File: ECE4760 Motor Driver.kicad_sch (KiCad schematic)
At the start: 48 parts, among them J1 IO, J100 Alternative Motor, J2 Motor / Power, J4 UART, U1 STM32G473V_B-C-E_Hx, U5 AP7361C-33FGE, U7 TPSM365R6, X1 48MHz

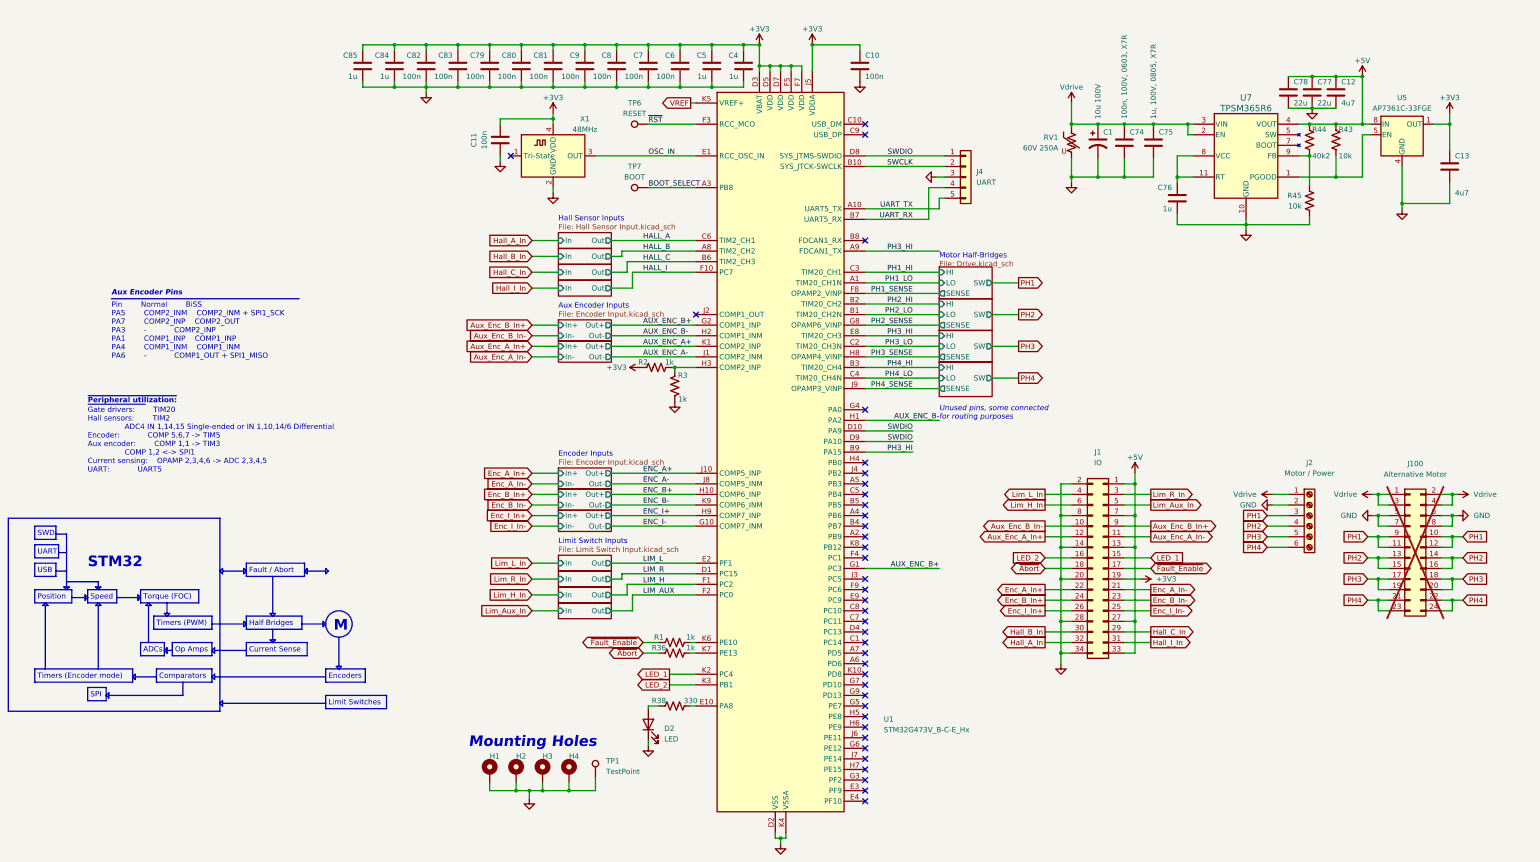
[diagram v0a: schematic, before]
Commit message: Ready for design review
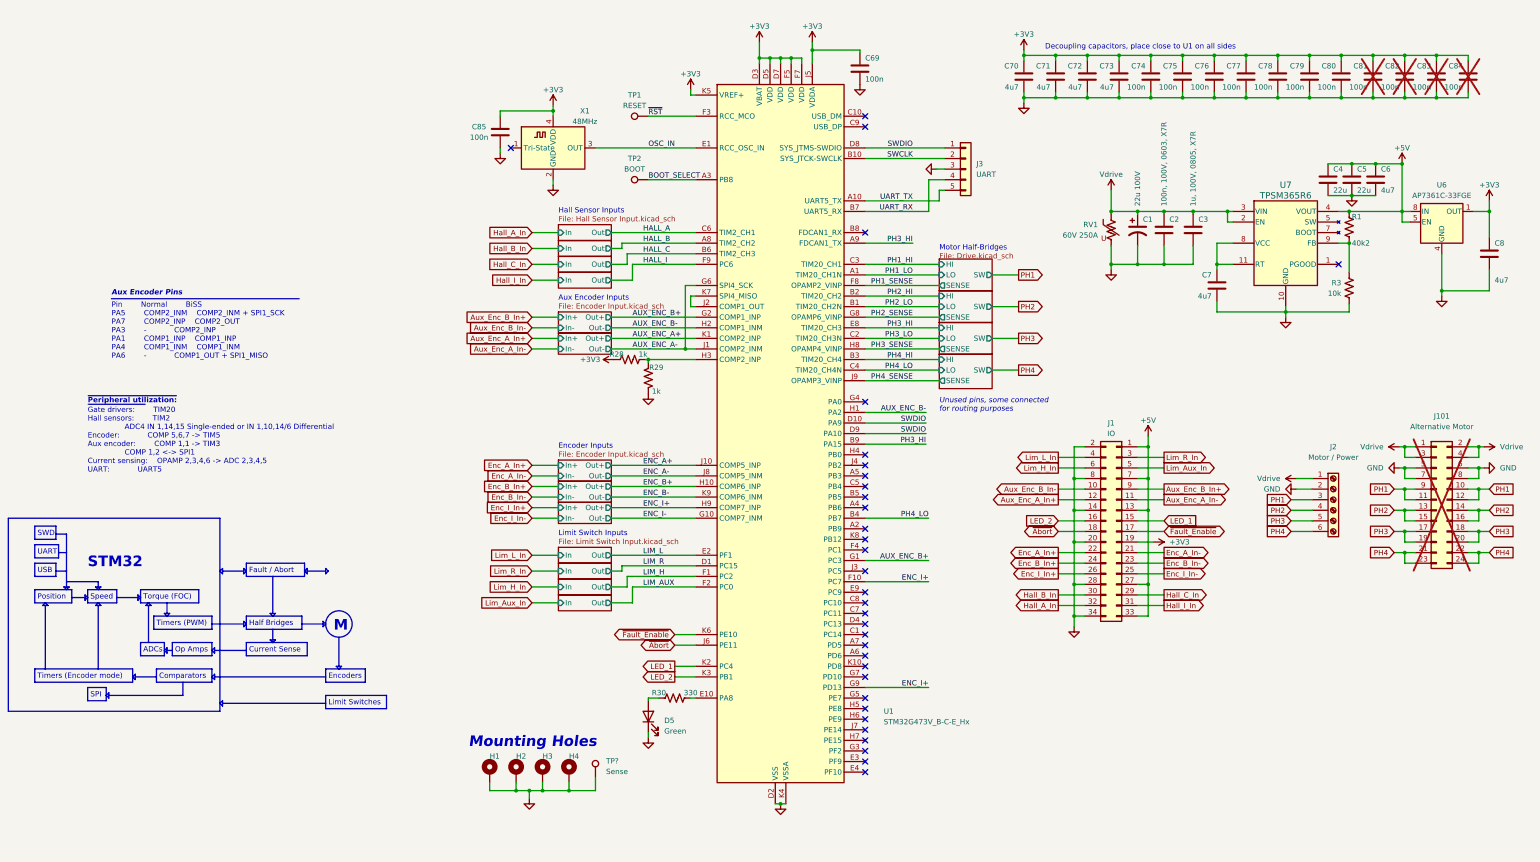
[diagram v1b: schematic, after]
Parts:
- removed R1, R36: 1k, Resistor_SMD:R_0402_1005Metric, symbol Device:R_US
- removed R43: 10k, Resistor_SMD:R_0402_1005Metric, symbol Device:R_US
- added C81, C82: 100n, Capacitor_SMD:C_0402_1005Metric, symbol Device:C
- C1: value 10u 100V -> 22u 100V
- C2: renamed from C74; DigiKey 490-3285-1-ND -> 490-13420-1-ND; LCSC (none) -> C161117
- C3: renamed from C75; LCSC (none) -> C5370002
- C4: renamed from C78; DigiKey (none) -> 490-GRM21BZ71A226ME15LCT-ND; LCSC (none) -> C907991
- C5: renamed from C77; DigiKey (none) -> 490-GRM21BZ71A226ME15LCT-ND; LCSC (none) -> C907991
- C6: renamed from C12; DigiKey (none) -> 490-GRM188Z71C475KE21DCT-ND; LCSC (none) -> C389010
- C69: renamed from C10; DigiKey 490-10700-1-ND -> 490-3261-1-ND; LCSC (none) -> C71629
- C7: renamed from C76; value 1u -> 4u7; DigiKey (none) -> 490-GRM188Z71C475KE21DCT-ND; LCSC (none) -> C389010
- C70: renamed from C5; value 1u -> 4u7; DigiKey (none) -> 490-GRM188Z71C475KE21DCT-ND; LCSC (none) -> C389010
- C71: renamed from C4; value 1u -> 4u7; DigiKey (none) -> 490-GRM188Z71C475KE21DCT-ND; LCSC (none) -> C389010
- C72: renamed from C85; value 1u -> 4u7; DigiKey (none) -> 490-GRM188Z71C475KE21DCT-ND; LCSC (none) -> C389010
- C73: renamed from C84; value 1u -> 4u7; DigiKey (none) -> 490-GRM188Z71C475KE21DCT-ND; LCSC (none) -> C389010
- C74: renamed from C79; DigiKey 490-10700-1-ND -> 490-3261-1-ND; LCSC (none) -> C71629
- C75: renamed from C80; DigiKey 490-10700-1-ND -> 490-3261-1-ND; LCSC (none) -> C71629
- C76: renamed from C81; DigiKey 490-10700-1-ND -> 490-3261-1-ND; LCSC (none) -> C71629
- C77: renamed from C9; DigiKey 490-10700-1-ND -> 490-3261-1-ND; LCSC (none) -> C71629
- C78: renamed from C8; DigiKey 490-10700-1-ND -> 490-3261-1-ND; LCSC (none) -> C71629
- C79: renamed from C7; DigiKey 490-10700-1-ND -> 490-3261-1-ND; LCSC (none) -> C71629
- C8: renamed from C13; DigiKey (none) -> 490-GRM188Z71C475KE21DCT-ND; LCSC (none) -> C389010
- C80: renamed from C6; DigiKey 490-10700-1-ND -> 490-3261-1-ND; LCSC (none) -> C71629
- C83: renamed from C82; DigiKey 490-10700-1-ND -> 490-3261-1-ND; LCSC (none) -> C71629; now not fitted; now left out of the parts list
- C84: renamed from C83; DigiKey 490-10700-1-ND -> 490-3261-1-ND; LCSC (none) -> C71629; now not fitted; now left out of the parts list
- C85: renamed from C11; DigiKey 490-10700-1-ND -> 490-3261-1-ND; LCSC (none) -> C71629
- D5: renamed from D2; value LED -> Green; DigiKey (none) -> 160-2018-1-ND; LCSC (none) -> C364563
- R1: renamed from R44; DigiKey 311-1.00KLRCT-ND -> 311-40.2KLRCT-ND; LCSC (none) -> C137983
- R28: renamed from R2; LCSC (none) -> C2935237
- R29: renamed from R3; LCSC (none) -> C2935237
- R3: renamed from R45; DigiKey 311-1.00KLRCT-ND -> 311-10.0KLRCT-ND; LCSC (none) -> C60490
- R30: renamed from R38; DigiKey (none) -> 311-330KLRCT-ND; LCSC (none) -> C138006
- TP1: renamed from TP6; now left out of the parts list
- TP2: renamed from TP7; now left out of the parts list
- TP?: renamed from TP1; value TestPoint -> Sense
- renumbered J100 to J101, J4 to J3, U5 to U6
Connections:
- net VREF is gone; now on net +3V3: U1.K5 (VREF+)
- net +3V3: now also C81.1, C82.1
- net +5V: now also U6.5 (EN)
- net AUX_ENC_A-: now also U1.G6 (PE12)
- net ENC_I+: now also U1.F10 (PC7), U1.G9 (PD13)
- net GND: now also C81.2, C82.2
- net HALL_I: now also U1.F9 (PC6); no longer U1.F10 (PC7)
- net PH4_LO: now also U1.B4 (PB7)
- net ~{Abort}: now also U1.J6 (PE11)
- net ~{Fault_Enable}: now also U1.K6 (PE10)
- net at U7.1 (PGOOD): no longer U6.5 (EN)
- net at U1.K7 (PE13): now also U1.J2 (PA6)
- no-connect marks 38 -> 33
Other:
- note added: "Decoupling capacitors, place close to U1 on all sides"
- moved on the sheet: C1, C2, C3, C4, C5, C6, C69, C7, C70, C71, C72, C73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
